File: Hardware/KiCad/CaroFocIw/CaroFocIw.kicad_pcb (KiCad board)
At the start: 4 copper layers, 85 x 42 mm, 100 parts, among them J1 Conn_01x04, J10 Conn_01x03, J11 Conn_01x03, J12 Conn_01x03, J13 Conn_01x04, J14 Conn_01x04, J15 Conn_01x04, J16 Conn_01x04, J17 Conn_01x04, J18 Conn_01x04, J19 Conn_01x02, J2 Conn_01x01, J20 Conn_01x02, J3 Conn_01x01, J4 Conn_01x04_MountingPin, J5 Conn_01x02, J6 Conn_01x02, J7 Conn_01x03, J8 Conn_01x03, J9 Conn_01x03, Q1 BSZ013NE2LS5I, Q2 BSZ013NE2LS5I, Q3 BSZ013NE2LS5I, Q4 BSZ013NE2LS5I, Q5 BSZ013NE2LS5I, Q6 BSZ013NE2LS5I, U1 Conn_01x01, U2 TCAN332, U3 STM32F405RGTx, U4 TLE7185-1E, U5 ACS711xEXLT-15AB, U6 AS5048A, U7 ACS711xEXLT-15AB, U8 ACS711xEXLT-15AB, U9 LMR16006YQ3

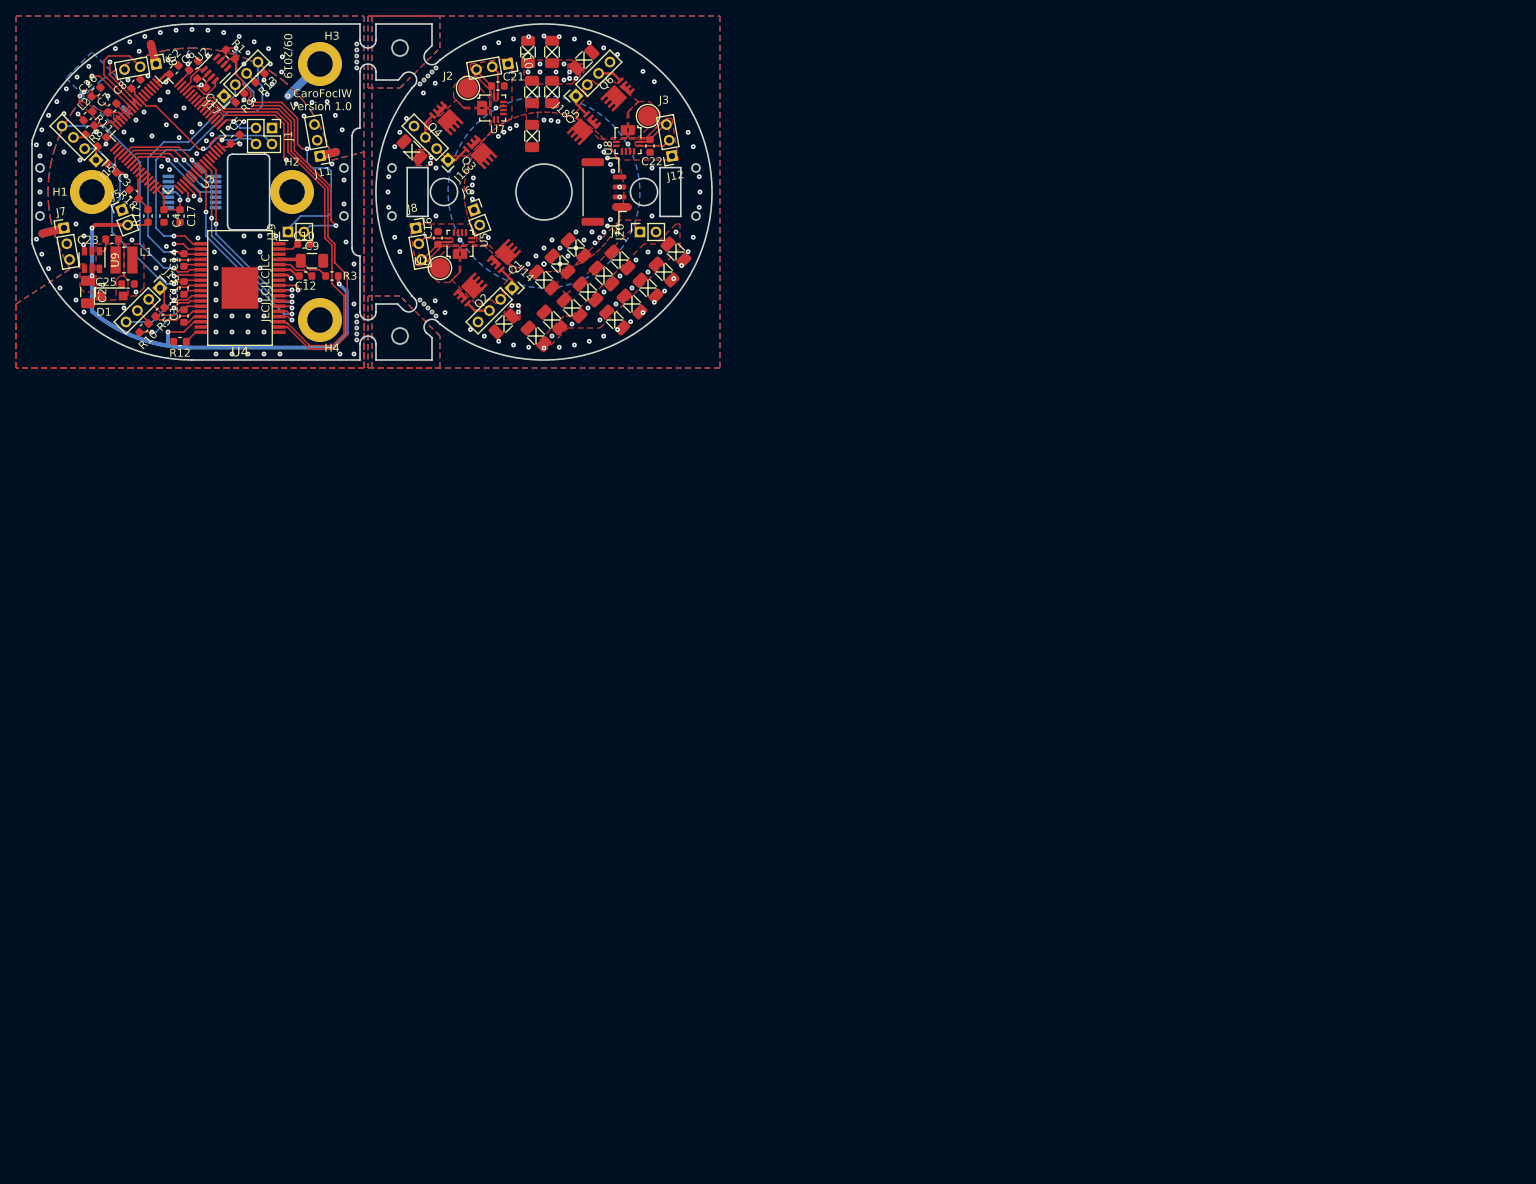
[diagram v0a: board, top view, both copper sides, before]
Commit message: documentation
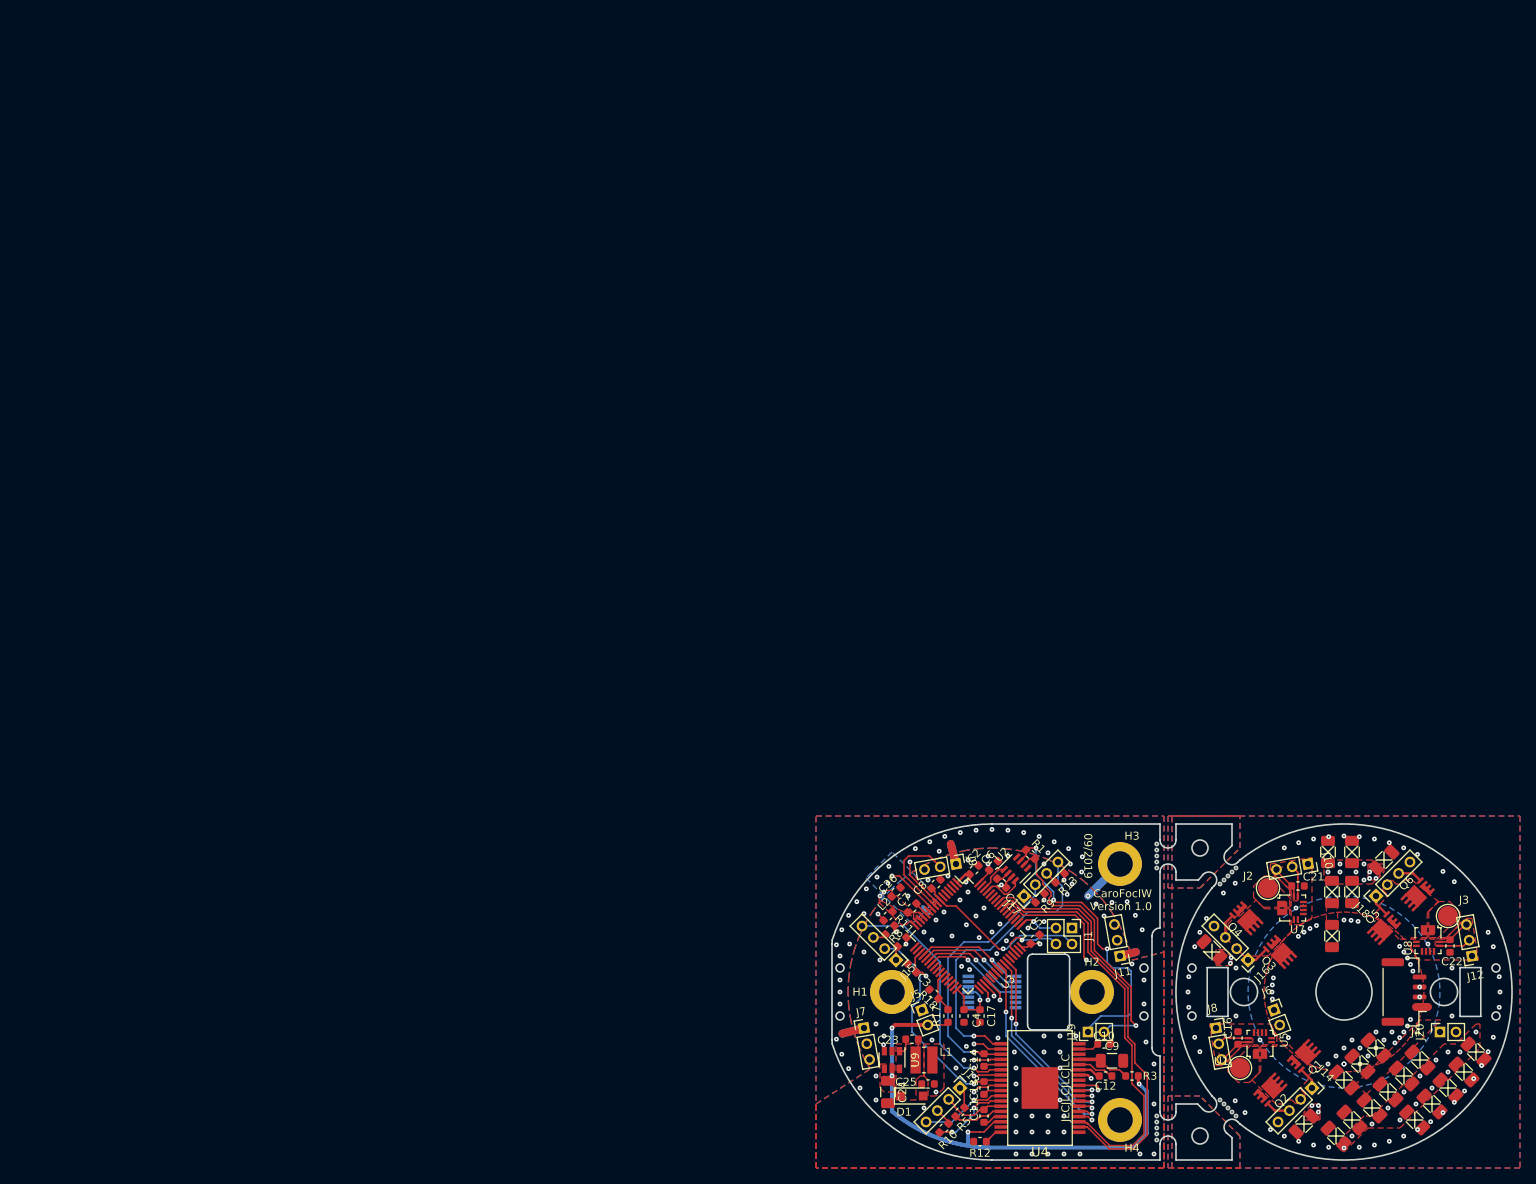
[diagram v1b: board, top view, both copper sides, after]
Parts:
- moved C1 141.4 mm to (101.2, 86.4)
- moved C10 141.4 mm to (114.0, 106.5)
- moved C11 141.4 mm to (99.0, 115.5)
- moved C12 141.4 mm to (114.2, 110.5)
- moved C13 141.4 mm to (99.0, 112.0)
- moved C14 141.4 mm to (99.0, 108.5)
- moved C15 141.4 mm to (139.0, 116.5)
- moved C16 141.4 mm to (130.8, 105.8)
- moved C17 141.4 mm to (98.5, 103.0)
- moved C19 141.4 mm to (127.5, 94.7)
- moved C2 141.4 mm to (97.8, 84.8)
- moved C20 141.4 mm to (149.0, 83.5)
- moved C21 141.4 mm to (138.2, 86.8)
- moved C22 141.4 mm to (157.2, 94.2)
- moved C23 141.4 mm to (90.0, 105.9)
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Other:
- outline, holes or cut-outs redrawn
